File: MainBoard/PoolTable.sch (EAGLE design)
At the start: 50 parts, among them IC6 LM317MBSTT3, M0 MOLEX-ULTRAFIT-1X03-VERT, M1 MOLEX-ULTRAFIT-1X03VERT, M2 MOLEX-ULTRAFIT-1X03VERT, M3 MOLEX-ULTRAFIT-1X03VERT, M4 MOLEX-ULTRAFIT-1X03VERT, M5 MOLEX-ULTRAFIT-1X03VERT, M6 MOLEX-ULTRAFIT-1X03VERT, M7 MOLEX-ULTRAFIT-1X03VERT, M8 MOLEX-ULTRAFIT-1X03-VERT, Q1 60V/32A/35mΩ, Q2 60V/32A/35mΩ, Q3 60V/32A/35mΩ, Q4 60V/32A/35mΩ, Q5 60V/32A/35mΩ, Q6 60V/32A/35mΩ, Q7 60V/32A/35mΩ, Q8 60V/32A/35mΩ, Q9 60V/32A/35mΩ, U1 TMP102, U2 TMP102, U3 TMP102, U4 TMP102

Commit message: Got a lot of routing done
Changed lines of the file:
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@@
 <?xml version="1.0" encoding="utf-8"?>
 <!DOCTYPE eagle SYSTEM "eagle.dtd">
-<eagle version="9.3.0">
+<eagle version="9.3.1">
 <drawing>
 <settings>
@@
 <part name="SUPPLY38" library="SparkFun-PowerSymbols" deviceset="12V" device=""/>
 <part name="SUPPLY39" library="SparkFun-PowerSymbols" deviceset="1.8V" device=""/>
-<part name="FRAME1" library="frames" library_urn="urn:adsk.eagle:library:229" deviceset="FRAME_C_L" device=""/>
 <part name="CPU0" library="Modules" deviceset="CPU_MODULE" device=""/>
 <part name="SUPPLY1" library="SparkFun-PowerSymbols" deviceset="3.3V" device=""/>
@@
 </nets>
 </sheet>
-<sheet>
-<plain>
-<text x="454.66" y="30.48" size="2.54" layer="94">Misc Components</text>
-<text x="546.1" y="7.62" size="2.54" layer="94">A</text>
-</plain>
-<instances>
-<instance part="FRAME1" gate="G$1" x="0" y="0" smashed="yes"/>
-<instance part="FRAME1" gate="G$2" x="452.12" y="0" smashed="yes">
-<attribute name="LAST_DATE_TIME" x="464.82" y="1.27" size="2.54" layer="94"/>
-<attribute name="SHEET" x="538.48" y="1.27" size="2.54" layer="94"/>
-<attribute name="DRAWING_NAME" x="469.9" y="19.05" size="2.54" layer="94"/>
-</instance>
-</instances>
-<busses>
-</busses>
-<nets>
-</nets>
-</sheet>

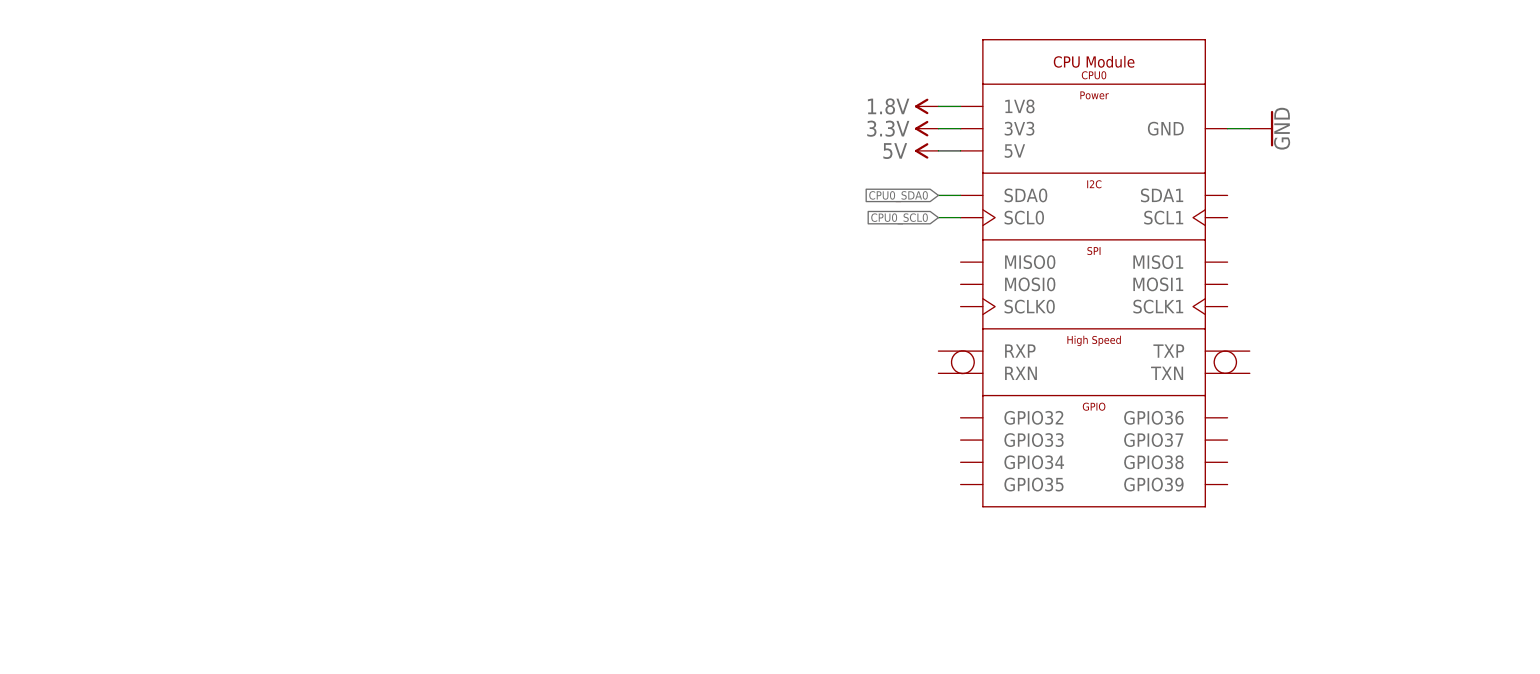
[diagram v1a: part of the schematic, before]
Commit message: latest
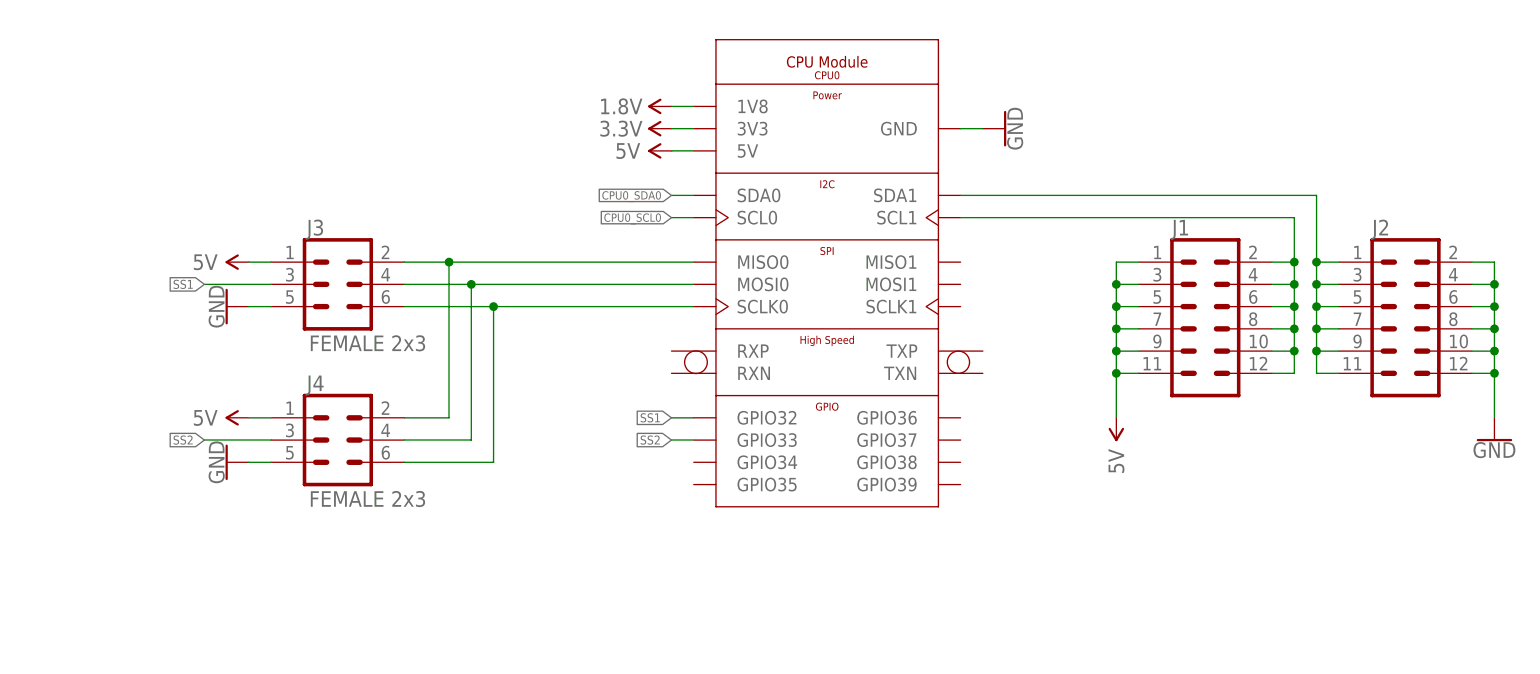
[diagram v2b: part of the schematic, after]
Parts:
- added J1, J2: 2X6 FEMALE, SparkFun-Connectors:CONN_06X2PTH_FEMALE
- added J3, J4: FEMALE 2x3, SparkFun-Connectors:CONN_03X2FEMALE
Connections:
- new net N$17: CPU0.MISO0, J3.2, J4.2
- new net N$18: CPU0.MOSI0, J3.4, J4.4
- new net N$19: CPU0.SCLK0, J3.6, J4.6
- new net N$4: CPU0.SCL1, J1.10, J1.12, J1.2, J1.4, J1.6, J1.8
- new net N$5: CPU0.SDA1, J2.1, J2.11, J2.3, J2.5, J2.7, J2.9
- new net SS1: CPU0.GPIO32, J3.3
- new net SS2: CPU0.GPIO33, J4.3
- net 5V: now also J1.1, J1.11, J1.3, J1.5, J1.7, J1.9, J3.1, J4.1
- net GND: now also J2.10, J2.12, J2.2, J2.4, J2.6, J2.8, J3.5, J4.5
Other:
- moved on the sheet: CPU0
